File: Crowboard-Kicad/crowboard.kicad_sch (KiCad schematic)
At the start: 73 parts, among them U1 Pico

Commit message: move
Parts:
- MX1, MX10, MX2, MX3, MX4, MX5, MX6, MX7, MX8, MX9: footprint Keebio-Parts:Kailh-PG1350-1u-NoLED -> (none)
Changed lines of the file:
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@@
       (effects (font (size 0.508 0.508)))
     )
-    (property "Footprint" "Keebio-Parts:Kailh-PG1350-1u-NoLED" (id 2) (at 154.305 55.245 0)
+    (property "Footprint" "" (id 2) (at 154.305 55.245 0)
       (effects (font (size 1.524 1.524)) hide)
     )
@@
       (effects (font (size 0.508 0.508)))
     )
-    (property "Footprint" "Keebio-Parts:Kailh-PG1350-1u-NoLED" (id 2) (at 188.595 55.245 0)
+    (property "Footprint" "" (id 2) (at 188.595 55.245 0)
       (effects (font (size 1.524 1.524)) hide)
     )
@@
       (effects (font (size 0.508 0.508)))
     )
-    (property "Footprint" "Keebio-Parts:Kailh-PG1350-1u-NoLED" (id 2) (at 142.875 55.245 0)
+    (property "Footprint" "" (id 2) (at 142.875 55.245 0)
       (effects (font (size 1.524 1.524)) hide)
     )
@@
       (effects (font (size 0.508 0.508)))
     )
-    (property "Footprint" "Keebio-Parts:Kailh-PG1350-1u-NoLED" (id 2) (at 222.885 55.245 0)
+    (property "Footprint" "" (id 2) (at 222.885 55.245 0)
       (effects (font (size 1.524 1.524)) hide)
     )
@@
       (effects (font (size 0.508 0.508)))
     )
-    (property "Footprint" "Keebio-Parts:Kailh-PG1350-1u-NoLED" (id 2) (at 131.445 55.245 0)
+    (property "Footprint" "" (id 2) (at 131.445 55.245 0)
       (effects (font (size 1.524 1.524)) hide)
     )
@@
       (effects (font (size 0.508 0.508)))
     )
-    (property "Footprint" "Keebio-Parts:Kailh-PG1350-1u-NoLED" (id 2) (at 120.015 55.245 0)
+    (property "Footprint" "" (id 2) (at 120.015 55.245 0)
       (effects (font (size 1.524 1.524)) hide)
     )
@@
       (effects (font (size 0.508 0.508)))
     )
-    (property "Footprint" "Keebio-Parts:Kailh-PG1350-1u-NoLED" (id 2) (at 177.165 55.245 0)
+    (property "Footprint" "" (id 2) (at 177.165 55.245 0)
       (effects (font (size 1.524 1.524)) hide)
     )
@@
       (effects (font (size 0.508 0.508)))
     )
-    (property "Footprint" "Keebio-Parts:Kailh-PG1350-1u-NoLED" (id 2) (at 165.735 55.245 0)
+    (property "Footprint" "" (id 2) (at 165.735 55.245 0)
       (effects (font (size 1.524 1.524)) hide)
     )
@@
       (effects (font (size 0.508 0.508)))
     )
-    (property "Footprint" "Keebio-Parts:Kailh-PG1350-1u-NoLED" (id 2) (at 200.025 55.245 0)
+    (property "Footprint" "" (id 2) (at 200.025 55.245 0)
       (effects (font (size 1.524 1.524)) hide)
     )
@@
       (effects (font (size 0.508 0.508)))
     )
-    (property "Footprint" "Keebio-Parts:Kailh-PG1350-1u-NoLED" (id 2) (at 211.455 55.245 0)
-      (effects (font (size 1.524 1.524)) hide)
-    )
+    (property "Footprint" "" (id 2) (at 211.455 55.245 0)
+      (effects (font (size 1.524 1.524)) hide)
+    )

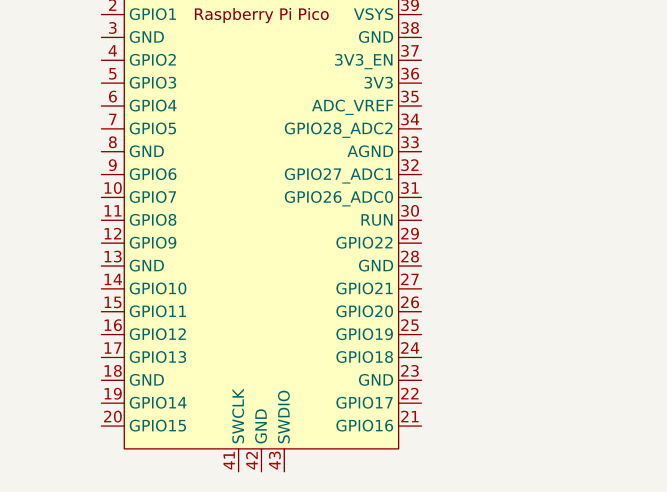
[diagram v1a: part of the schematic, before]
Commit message: finished
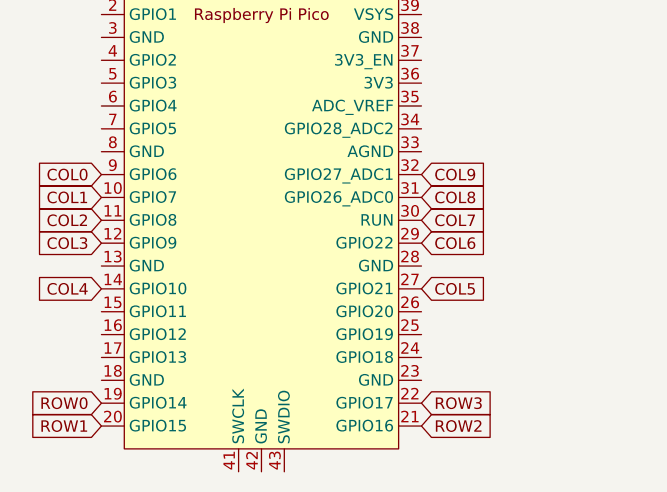
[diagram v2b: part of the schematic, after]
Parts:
- MX1, MX10, MX2, MX3, MX4, MX5, MX6, MX7, MX8, MX9: footprint (none) -> Keebio-Parts:Kailh-PG1350-1u-NoLED
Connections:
- net COL0: now also U1.9 (GPIO6)
- net COL1: now also U1.10 (GPIO7)
- net COL2: now also U1.11 (GPIO8)
- net COL3: now also U1.12 (GPIO9)
- net COL4: now also U1.14 (GPIO10)
- net COL5: now also U1.27 (GPIO21)
- net COL6: now also U1.29 (GPIO22)
- net COL7: now also U1.30 (RUN)
- net COL8: now also U1.31 (GPIO26_ADC0)
- net COL9: now also U1.32 (GPIO27_ADC1)
- net ROW0: now also U1.19 (GPIO14)
- net ROW1: now also U1.20 (GPIO15)
- net ROW2: now also U1.21 (GPIO16)
- net ROW3: now also U1.22 (GPIO17)
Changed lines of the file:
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@@
     (stroke (width 0) (type default) (color 0 0 0 0))
   )
+  (global_label "COL9" (shape input) (at 76.2 92.71 0) (fields_autoplaced)
+    (effects (font (size 1.27 1.27)) (justify left))
+    (property "Intersheet References" "${INTERSHEET_REFS}" (id 0) (at 83.4512 92.6306 0)
+      (effects (font (size 1.27 1.27)) (justify left) hide)
+    )
+  )
   (global_label "ROW2" (shape input) (at 128.27 99.06 180) (fields_autoplaced)
     (effects (font (size 1.27 1.27)) (justify right))
@@
     )
   )
+  (global_label "COL1" (shape input) (at 40.64 95.25 180) (fields_autoplaced)
+    (effects (font (size 1.27 1.27)) (justify right))
+    (property "Intersheet References" "${INTERSHEET_REFS}" (id 0) (at 33.3888 95.1706 0)
+      (effects (font (size 1.27 1.27)) (justify right) hide)
+    )
+  )
   (global_label "COL5" (shape input) (at 196.85 43.18 90) (fields_autoplaced)
     (effects (font (size 1.27 1.27)) (justify left))
@@
     )
   )
+  (global_label "COL2" (shape input) (at 40.64 97.79 180) (fields_autoplaced)
+    (effects (font (size 1.27 1.27)) (justify right))
+    (property "Intersheet References" "${INTERSHEET_REFS}" (id 0) (at 33.3888 97.7106 0)
+      (effects (font (size 1.27 1.27)) (justify right) hide)
+    )
+  )
   (global_label "COL6" (shape input) (at 208.28 43.18 90) (fields_autoplaced)
     (effects (font (size 1.27 1.27)) (justify left))
@@
     )
   )
+  (global_label "COL6" (shape input) (at 76.2 100.33 0) (fields_autoplaced)
+    (effects (font (size 1.27 1.27)) (justify left))
+    (property "Intersheet References" "${INTERSHEET_REFS}" (id 0) (at 83.4512 100.2506 0)
+      (effects (font (size 1.27 1.27)) (justify left) hide)
+    )
+  )
   (global_label "COL9" (shape input) (at 242.57 43.18 90) (fields_autoplaced)
     (effects (font (size 1.27 1.27)) (justify left))
@@
     )
   )
+  (global_label "ROW3" (shape input) (at 76.2 118.11 0) (fields_autoplaced)
+    (effects (font (size 1.27 1.27)) (justify left))
+    (property "Intersheet References" "${INTERSHEET_REFS}" (id 0) (at 83.8745 118.0306 0)
+      (effects (font (size 1.27 1.27)) (justify left) hide)
+    )
+  )
+  (global_label "COL7" (shape input) (at 76.2 97.79 0) (fields_autoplaced)
+    (effects (font (size 1.27 1.27)) (justify left))
+    (property "Intersheet References" "${INTERSHEET_REFS}" (id 0) (at 83.4512 97.7106 0)
+      (effects (font (size 1.27 1.27)) (justify left) hide)
+    )
+  )
+  (global_label "COL8" (shape input) (at 76.2 95.25 0) (fields_autoplaced)
+    (effects (font (size 1.27 1.27)) (justify left))
+    (property "Intersheet References" "${INTERSHEET_REFS}" (id 0) (at 83.4512 95.1706 0)
+      (effects (font (size 1.27 1.27)) (justify left) hide)
+    )
+  )
   (global_label "COL1" (shape input) (at 151.13 43.18 90) (fields_autoplaced)
     (effects (font (size 1.27 1.27)) (justify left))
@@
     )
   )
+  (global_label "COL3" (shape input) (at 40.64 100.33 180) (fields_autoplaced)
+    (effects (font (size 1.27 1.27)) (justify right))
+    (property "Intersheet References" "${INTERSHEET_REFS}" (id 0) (at 33.3888 100.2506 0)
+      (effects (font (size 1.27 1.27)) (justify right) hide)
+    )
+  )
+  (global_label "ROW2" (shape input) (at 76.2 120.65 0) (fields_autoplaced)
+    (effects (font (size 1.27 1.27)) (justify left))
+    (property "Intersheet References" "${INTERSHEET_REFS}" (id 0) (at 83.8745 120.5706 0)
+      (effects (font (size 1.27 1.27)) (justify left) hide)
+    )
+  )
   (global_label "ROW1" (shape input) (at 128.27 81.28 180) (fields_autoplaced)
     (effects (font (size 1.27 1.27)) (justify right))
@@
     )
   )
+  (global_label "COL5" (shape input) (at 76.2 105.41 0) (fields_autoplaced)
+    (effects (font (size 1.27 1.27)) (justify left))
+    (property "Intersheet References" "${INTERSHEET_REFS}" (id 0) (at 83.4512 105.3306 0)
+      (effects (font (size 1.27 1.27)) (justify left) hide)
+    )
+  )
   (global_label "COL4" (shape input) (at 185.42 43.18 90) (fields_autoplaced)
     (effects (font (size 1.27 1.27)) (justify left))
@@
     )
   )
+  (global_label "ROW1" (shape input) (at 40.64 120.65 180) (fields_autoplaced)
+    (effects (font (size 1.27 1.27)) (justify right))
+    (property "Intersheet References" "${INTERSHEET_REFS}" (id 0) (at 32.9655 120.5706 0)
+      (effects (font (size 1.27 1.27)) (justify right) hide)
+    )
+  )
   (global_label "ROW0" (shape input) (at 128.27 63.5 180) (fields_autoplaced)
     (effects (font (size 1.27 1.27)) (justify right))
@@
     )
   )
+  (global_label "COL0" (shape input) (at 40.64 92.71 180) (fields_autoplaced)
+    (effects (font (size 1.27 1.27)) (justify right))
+    (property "Intersheet References" "${INTERSHEET_REFS}" (id 0) (at 33.3888 92.6306 0)
+      (effects (font (size 1.27 1.27)) (justify right) hide)
+    )
+  )
   (global_label "ROW3" (shape input) (at 144.78 116.84 180) (fields_autoplaced)
     (effects (font (size 1.27 1.27)) (justify right))
@@
     )
   )
+  (global_label "ROW0" (shape input) (at 40.64 118.11 180) (fields_autoplaced)
+    (effects (font (size 1.27 1.27)) (justify right))
+    (property "Intersheet References" "${INTERSHEET_REFS}" (id 0) (at 32.9655 118.0306 0)
+      (effects (font (size 1.27 1.27)) (justify right) hide)
+    )
+  )
+  (global_label "COL4" (shape input) (at 40.64 105.41 180) (fields_autoplaced)
+    (effects (font (size 1.27 1.27)) (justify right))
+    (property "Intersheet References" "${INTERSHEET_REFS}" (id 0) (at 33.3888 105.3306 0)
+      (effects (font (size 1.27 1.27)) (justify right) hide)
+    )
+  )
   (global_label "COL7" (shape input) (at 219.71 43.18 90) (fields_autoplaced)
     (effects (font (size 1.27 1.27)) (justify left))
@@
       (effects (font (size 0.508 0.508)))
     )
-    (property "Footprint" "" (id 2) (at 154.305 55.245 0)
+    (property "Footprint" "Keebio-Parts:Kailh-PG1350-1u-NoLED" (id 2) (at 154.305 55.245 0)
       (effects (font (size 1.524 1.524)) hide)
     )
@@
       (effects (font (size 0.508 0.508)))
     )
-    (property "Footprint" "" (id 2) (at 188.595 55.245 0)
+    (property "Footprint" "Keebio-Parts:Kailh-PG1350-1u-NoLED" (id 2) (at 188.595 55.245 0)
       (effects (font (size 1.524 1.524)) hide)
     )
@@
       (effects (font (size 0.508 0.508)))
     )
-    (property "Footprint" "" (id 2) (at 142.875 55.245 0)
+    (property "Footprint" "Keebio-Parts:Kailh-PG1350-1u-NoLED" (id 2) (at 142.875 55.245 0)
       (effects (font (size 1.524 1.524)) hide)
     )
@@
       (effects (font (size 0.508 0.508)))
     )
-    (property "Footprint" "" (id 2) (at 222.885 55.245 0)
+    (property "Footprint" "Keebio-Parts:Kailh-PG1350-1u-NoLED" (id 2) (at 222.885 55.245 0)
       (effects (font (size 1.524 1.524)) hide)
     )
@@
       (effects (font (size 0.508 0.508)))
     )
-    (property "Footprint" "" (id 2) (at 131.445 55.245 0)
+    (property "Footprint" "Keebio-Parts:Kailh-PG1350-1u-NoLED" (id 2) (at 131.445 55.245 0)
       (effects (font (size 1.524 1.524)) hide)
     )
@@
       (effects (font (size 0.508 0.508)))
     )
-    (property "Footprint" "" (id 2) (at 120.015 55.245 0)
+    (property "Footprint" "Keebio-Parts:Kailh-PG1350-1u-NoLED" (id 2) (at 120.015 55.245 0)
       (effects (font (size 1.524 1.524)) hide)
     )
@@
       (effects (font (size 0.508 0.508)))
     )
-    (property "Footprint" "" (id 2) (at 177.165 55.245 0)
+    (property "Footprint" "Keebio-Parts:Kailh-PG1350-1u-NoLED" (id 2) (at 177.165 55.245 0)
       (effects (font (size 1.524 1.524)) hide)
     )
@@
       (effects (font (size 0.508 0.508)))
     )
-    (property "Footprint" "" (id 2) (at 165.735 55.245 0)
+    (property "Footprint" "Keebio-Parts:Kailh-PG1350-1u-NoLED" (id 2) (at 165.735 55.245 0)
       (effects (font (size 1.524 1.524)) hide)
     )
@@
       (effects (font (size 0.508 0.508)))
     )
-    (property "Footprint" "" (id 2) (at 200.025 55.245 0)
+    (property "Footprint" "Keebio-Parts:Kailh-PG1350-1u-NoLED" (id 2) (at 200.025 55.245 0)
       (effects (font (size 1.524 1.524)) hide)
     )
@@
       (effects (font (size 0.508 0.508)))
     )
-    (property "Footprint" "" (id 2) (at 211.455 55.245 0)
-      (effects (font (size 1.524 1.524)) hide)
-    )
+    (property "Footprint" "Keebio-Parts:Kailh-PG1350-1u-NoLED" (id 2) (at 211.455 55.245 0)
+      (effects (font (size 1.524 1.524)) hide)
+    )

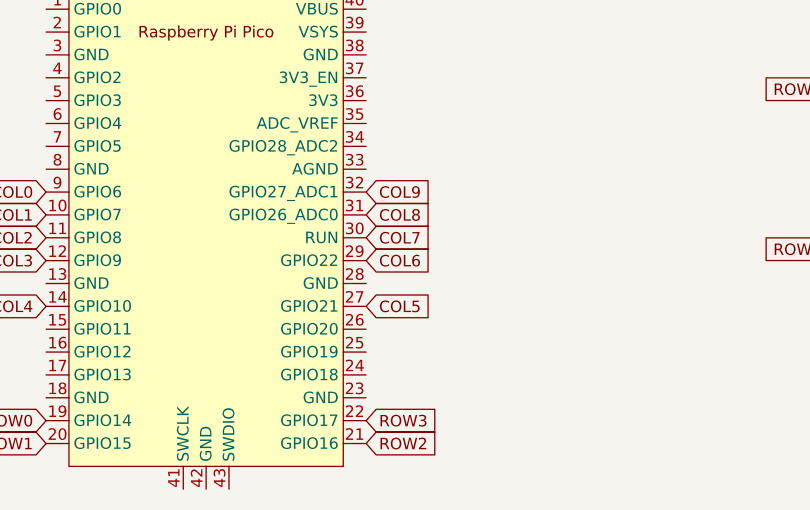
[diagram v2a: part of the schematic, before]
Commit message: fix routing
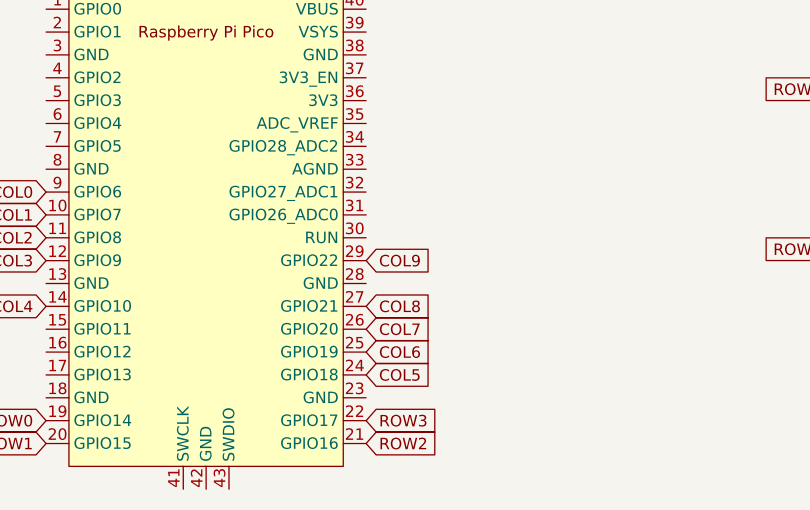
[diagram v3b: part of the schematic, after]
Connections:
- net COL5: now also U1.24 (GPIO18); no longer U1.27 (GPIO21)
- net COL6: now also U1.25 (GPIO19); no longer U1.29 (GPIO22)
- net COL7: now also U1.26 (GPIO20); no longer U1.30 (RUN)
- net COL8: now also U1.27 (GPIO21); no longer U1.31 (GPIO26_ADC0)
- net COL9: now also U1.29 (GPIO22); no longer U1.32 (GPIO27_ADC1)
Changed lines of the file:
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@@
     (stroke (width 0) (type default) (color 0 0 0 0))
   )
-  (global_label "COL9" (shape input) (at 76.2 92.71 0) (fields_autoplaced)
+  (global_label "COL9" (shape input) (at 76.2 100.33 0) (fields_autoplaced)
     (effects (font (size 1.27 1.27)) (justify left))
-    (property "Intersheet References" "${INTERSHEET_REFS}" (id 0) (at 83.4512 92.6306 0)
+    (property "Intersheet References" "${INTERSHEET_REFS}" (id 0) (at 83.4512 100.2506 0)
       (effects (font (size 1.27 1.27)) (justify left) hide)
     )
@@
     )
   )
-  (global_label "COL6" (shape input) (at 76.2 100.33 0) (fields_autoplaced)
+  (global_label "COL6" (shape input) (at 76.2 110.49 0) (fields_autoplaced)
     (effects (font (size 1.27 1.27)) (justify left))
-    (property "Intersheet References" "${INTERSHEET_REFS}" (id 0) (at 83.4512 100.2506 0)
+    (property "Intersheet References" "${INTERSHEET_REFS}" (id 0) (at 83.4512 110.4106 0)
       (effects (font (size 1.27 1.27)) (justify left) hide)
     )
@@
     )
   )
-  (global_label "COL7" (shape input) (at 76.2 97.79 0) (fields_autoplaced)
+  (global_label "COL7" (shape input) (at 76.2 107.95 0) (fields_autoplaced)
     (effects (font (size 1.27 1.27)) (justify left))
-    (property "Intersheet References" "${INTERSHEET_REFS}" (id 0) (at 83.4512 97.7106 0)
+    (property "Intersheet References" "${INTERSHEET_REFS}" (id 0) (at 83.4512 107.8706 0)
       (effects (font (size 1.27 1.27)) (justify left) hide)
     )
   )
-  (global_label "COL8" (shape input) (at 76.2 95.25 0) (fields_autoplaced)
+  (global_label "COL8" (shape input) (at 76.2 105.41 0) (fields_autoplaced)
     (effects (font (size 1.27 1.27)) (justify left))
-    (property "Intersheet References" "${INTERSHEET_REFS}" (id 0) (at 83.4512 95.1706 0)
+    (property "Intersheet References" "${INTERSHEET_REFS}" (id 0) (at 83.4512 105.3306 0)
       (effects (font (size 1.27 1.27)) (justify left) hide)
     )
@@
     )
   )
-  (global_label "COL5" (shape input) (at 76.2 105.41 0) (fields_autoplaced)
+  (global_label "COL5" (shape input) (at 76.2 113.03 0) (fields_autoplaced)
     (effects (font (size 1.27 1.27)) (justify left))
-    (property "Intersheet References" "${INTERSHEET_REFS}" (id 0) (at 83.4512 105.3306 0)
+    (property "Intersheet References" "${INTERSHEET_REFS}" (id 0) (at 83.4512 112.9506 0)
       (effects (font (size 1.27 1.27)) (justify left) hide)
     )
